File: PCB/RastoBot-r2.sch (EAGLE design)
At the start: 354 parts, among them IC1 PIC24FJ32GA002-X, Q1 FDD4141TO252, Q8 FDD4141TO252, T2 2N2222A, U1 PIC18F47J13-I/PT, U10 140357145000, U11 140357145000, U12 140357145000, U13 140357145000, U15 PIC32MK1024MCM064-I/PTTQFP64_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, U2 LIS3MDLTR, U4 140357145000, U5 MPU-6050, U6 140357145000, U7 140357145000, U8 140357145000, U9 140357145000, X5 FPS009-3000

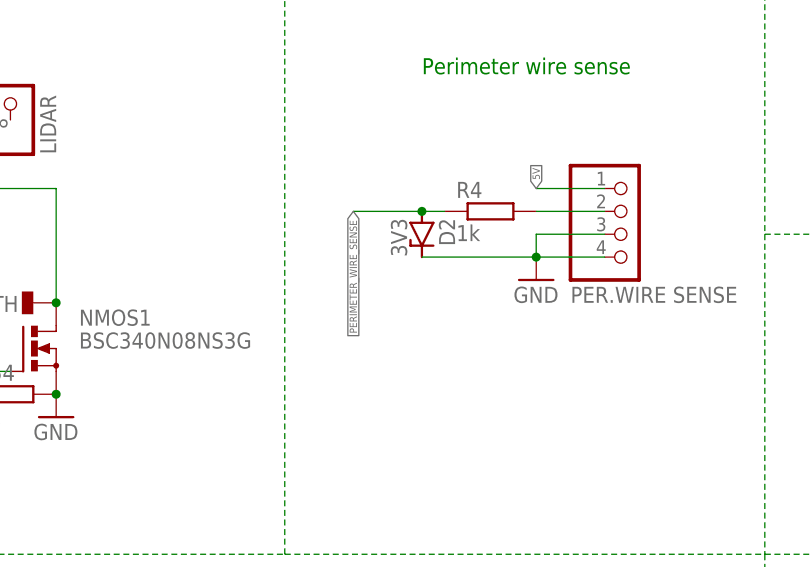
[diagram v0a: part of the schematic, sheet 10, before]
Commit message: GPS
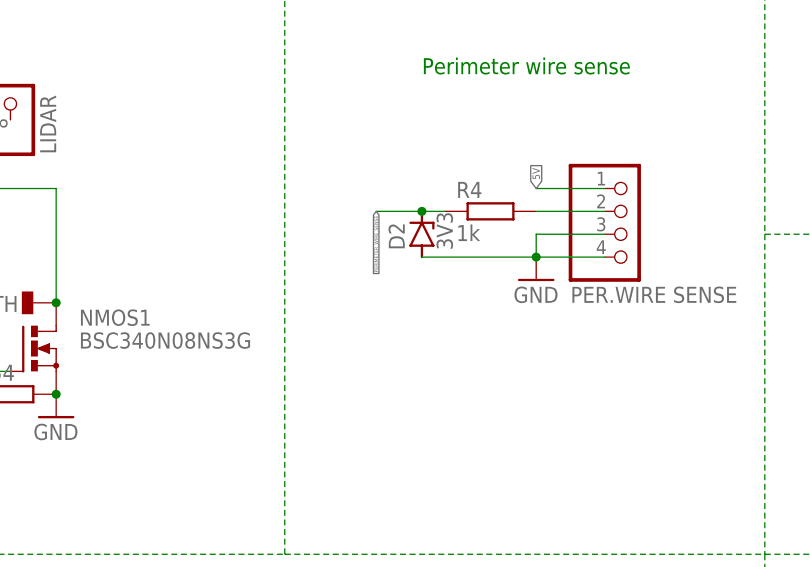
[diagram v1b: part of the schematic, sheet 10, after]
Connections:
- net GND: now also D2.A; no longer D2.C
- net PERIMETER_WIRE_SENSE: now also D2.C; no longer D2.A
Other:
- moved on the sheet: D2
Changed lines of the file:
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@@
 <attribute name="VALUE" x="102.87" y="108.458" size="1.778" layer="96"/>
 </instance>
-<instance part="D2" gate="G$1" x="99.06" y="109.22" smashed="yes" rot="R270">
-<attribute name="NAME" x="100.965" y="110.998" size="1.778" layer="95" rot="R270"/>
-<attribute name="VALUE" x="95.631" y="110.998" size="1.778" layer="96" rot="R270"/>
+<instance part="D2" gate="G$1" x="99.06" y="109.22" smashed="yes" rot="R90">
+<attribute name="NAME" x="97.155" y="107.442" size="1.778" layer="95" rot="R90"/>
+<attribute name="VALUE" x="102.489" y="107.442" size="1.778" layer="96" rot="R90"/>
 </instance>
 <instance part="LIGHT_SENSOR" gate="G$1" x="226.06" y="162.56" smashed="yes">
@@
 <wire x1="111.76" y1="109.22" x2="111.76" y2="106.68" width="0.1524" layer="91"/>
 <junction x="111.76" y="106.68"/>
-<pinref part="D2" gate="G$1" pin="C"/>
+<pinref part="D2" gate="G$1" pin="A"/>
 <wire x1="99.06" y1="106.68" x2="111.76" y2="106.68" width="0.1524" layer="91"/>
 </segment>
@@
 </segment>
 </net>
-<net name="PERIMETER_WIRE_SENSE" class="0">
-<segment>
-<pinref part="R4" gate="G$1" pin="1"/>
-<pinref part="D2" gate="G$1" pin="A"/>
-<wire x1="99.06" y1="111.76" x2="101.6" y2="111.76" width="0.1524" layer="91"/>
-<wire x1="99.06" y1="111.76" x2="91.44" y2="111.76" width="0.1524" layer="91"/>
-<junction x="99.06" y="111.76"/>
-<label x="91.44" y="111.76" size="0.8128" layer="95" rot="R270" xref="yes"/>
-</segment>
-</net>
 <net name="MCU_0_LIGHT_SENSOR" class="0">
 <segment>
@@
 </segment>
 </net>
+<net name="PERIMETER_WIRE_SENSE" class="0">
+<segment>
+<pinref part="D2" gate="G$1" pin="C"/>
+<pinref part="R4" gate="G$1" pin="1"/>
+<wire x1="99.06" y1="111.76" x2="101.6" y2="111.76" width="0.1524" layer="91"/>
+<wire x1="99.06" y1="111.76" x2="93.98" y2="111.76" width="0.1524" layer="91"/>
+<junction x="99.06" y="111.76"/>
+<label x="93.98" y="111.76" size="0.4064" layer="95" rot="R270" xref="yes"/>
+</segment>
+</net>
